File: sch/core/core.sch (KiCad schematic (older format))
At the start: 1 part, among them U1 STM32F427VITx

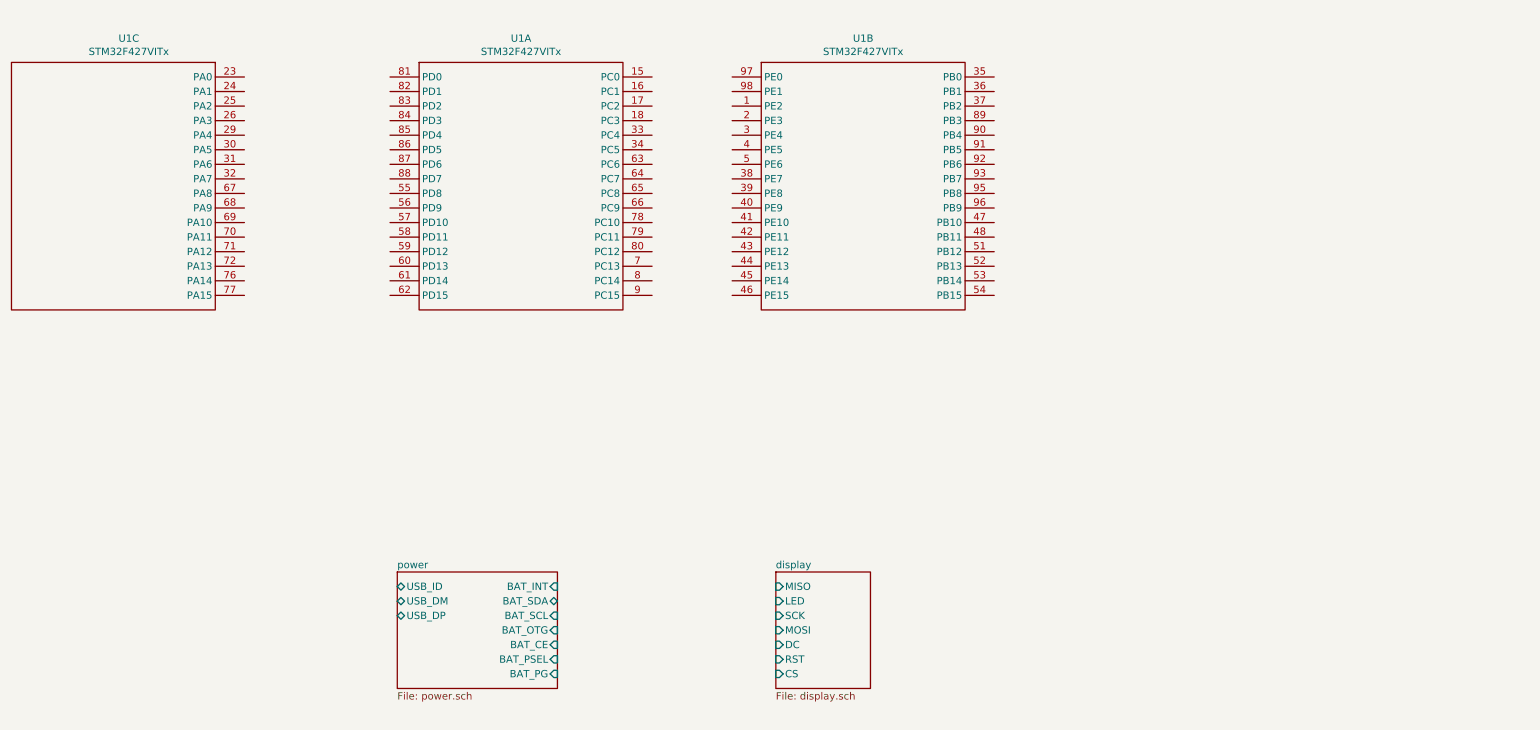
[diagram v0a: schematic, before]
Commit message: sch core done
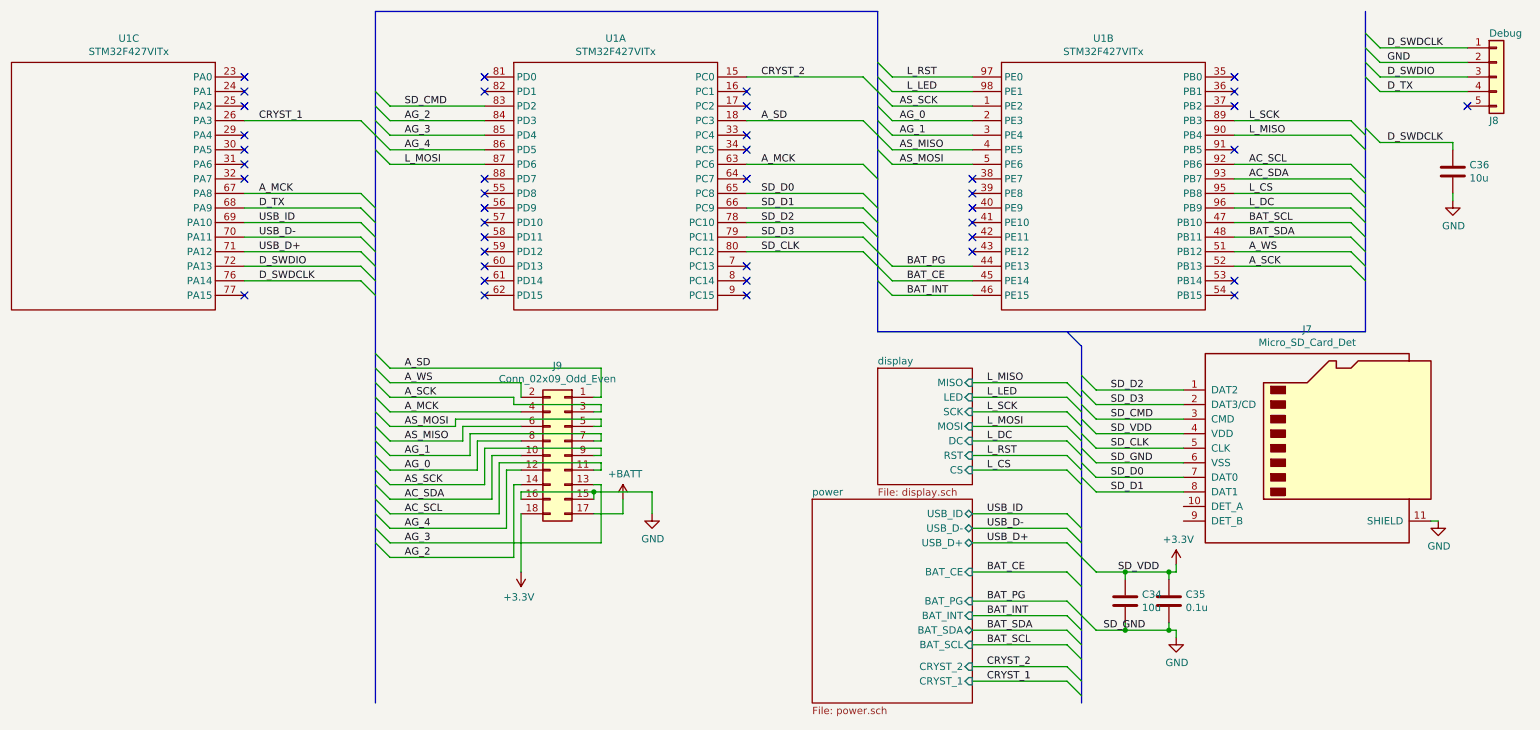
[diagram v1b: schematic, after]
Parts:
- added C34, C36: 10u, Capacitors_SMD:C_0805, symbol Device:C
- added C35: 0.1u, Capacitors_SMD:C_0402, symbol Device:C
- added J7: Micro_SD_Card_Det, Connectors_Hirose:microSD_Card_Receptacle_Hirose_DM3AT-SF-PEJM5, symbol Connector:Micro_SD_Card_Det
- added J8: Debug, Connector_PinHeader_1.27mm:PinHeader_1x05_P1.27mm_Vertical, symbol Connector_Generic:Conn_01x05
- added J9: Conn_02x09_Odd_Even, Connector_PinSocket_2.54mm:PinSocket_2x09_P2.54mm_Vertical, symbol Connector_Generic:Conn_02x09_Odd_Even
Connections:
- net CRYST_2: now reaches U1.15 (PC0)
- net A_SD: now reaches U1.18 (PC3)
- net A_SD: now also J9.1 (Pin_1)
- net A_MCK: now reaches U1.63 (PC6)
- net A_MCK: now also U1.67 (PA8), J9.4 (Pin_4)
- net SD_D0: now reaches U1.65 (PC8)
- net SD_D0: now also J7.7 (DAT0)
- net SD_D1: now reaches U1.66 (PC9)
- net SD_D1: now also J7.8 (DAT1)
- net SD_D2: now reaches U1.78 (PC10)
- net SD_D2: now also J7.1 (DAT2)
- net SD_D3: now reaches U1.79 (PC11)
- net SD_D3: now also J7.2 (DAT3/CD)
- net SD_CLK: now reaches U1.80 (PC12)
- net SD_CLK: now also J7.5 (CLK)
- net SD_CMD: now reaches U1.83 (PD2)
- net SD_CMD: now also J7.3 (CMD)
- net AG_2: now reaches U1.84 (PD3)
- net AG_2: now also J9.14 (Pin_14)
- net AG_3: now reaches U1.85 (PD4)
- net AG_3: now also J9.13 (Pin_13)
- net AG_4: now reaches U1.86 (PD5)
- net AG_4: now also J9.12 (Pin_12)
- net L_MOSI: now reaches U1.87 (PD6)
- net AS_SCK: now reaches U1.1 (PE2)
- net AS_SCK: now also J9.9 (Pin_9)
- net AG_0: now reaches U1.2 (PE3)
- net AG_0: now also J9.8 (Pin_8)
- net AG_1: now reaches U1.3 (PE4)
- net AG_1: now also J9.7 (Pin_7)
- net AS_MISO: now reaches U1.4 (PE5)
- net AS_MISO: now also J9.6 (Pin_6)
- net BAT_PG: now reaches U1.44 (PE13)
- net BAT_CE: now reaches U1.45 (PE14)
- net BAT_INT: now reaches U1.46 (PE15)
- net BAT_SCL: now reaches U1.47 (PB10)
- net BAT_SDA: now reaches U1.48 (PB11)
- net AS_MOSI: now reaches U1.5 (PE6)
- net AS_MOSI: now also J9.5 (Pin_5)
- net A_WS: now reaches U1.51 (PB12)
- net A_WS: now also J9.2 (Pin_2)
- net A_SCK: now reaches U1.52 (PB13)
- net A_SCK: now also J9.3 (Pin_3)
- net L_SCK: now reaches U1.89 (PB3)
- net L_MISO: now reaches U1.90 (PB4)
- net AC_SCL: now reaches U1.92 (PB6)
- net AC_SCL: now also J9.11 (Pin_11)
- net AC_SDA: now reaches U1.93 (PB7)
- net AC_SDA: now also J9.10 (Pin_10)
- net L_CS: now reaches U1.95 (PB8)
- net L_DC: now reaches U1.96 (PB9)
- net L_RST: now reaches U1.97 (PE0)
- net L_LED: now reaches U1.98 (PE1)
- net CRYST_1: now reaches U1.26 (PA3)
- net D_TX: now reaches U1.68 (PA9)
- net D_TX: now also J8.4 (Pin_4)
- net USB_ID: now reaches U1.69 (PA10)
- net USB_D-: now reaches U1.70 (PA11)
- net USB_D+: now reaches U1.71 (PA12)
- net D_SWDIO: now reaches U1.72 (PA13)
- net D_SWDIO: now also J8.3 (Pin_3)
- net D_SWDCLK: now reaches U1.76 (PA14)
- net D_SWDCLK: now also C36.1, J8.1 (Pin_1)
- new net +3V3: C34.1, C35.1, J7.4 (VDD), J9.18 (Pin_18)
- new net +BATT: J9.17 (Pin_17)
- new net GND: C34.2, C35.2, C36.2, J7.11 (SHIELD), J7.6 (VSS), J8.2 (Pin_2), J9.15 (Pin_15), J9.16 (Pin_16)
- no-connect marks 0 -> 40
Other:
- moved on the sheet: U1A, U1B
